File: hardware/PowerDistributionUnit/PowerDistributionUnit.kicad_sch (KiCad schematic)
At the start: 52 parts, among them J1 973582101, J2 973582100, J3 973582101, J4 973582100, Q16 CSD18511Q5A, U1 TPS25983, U2 AD5258

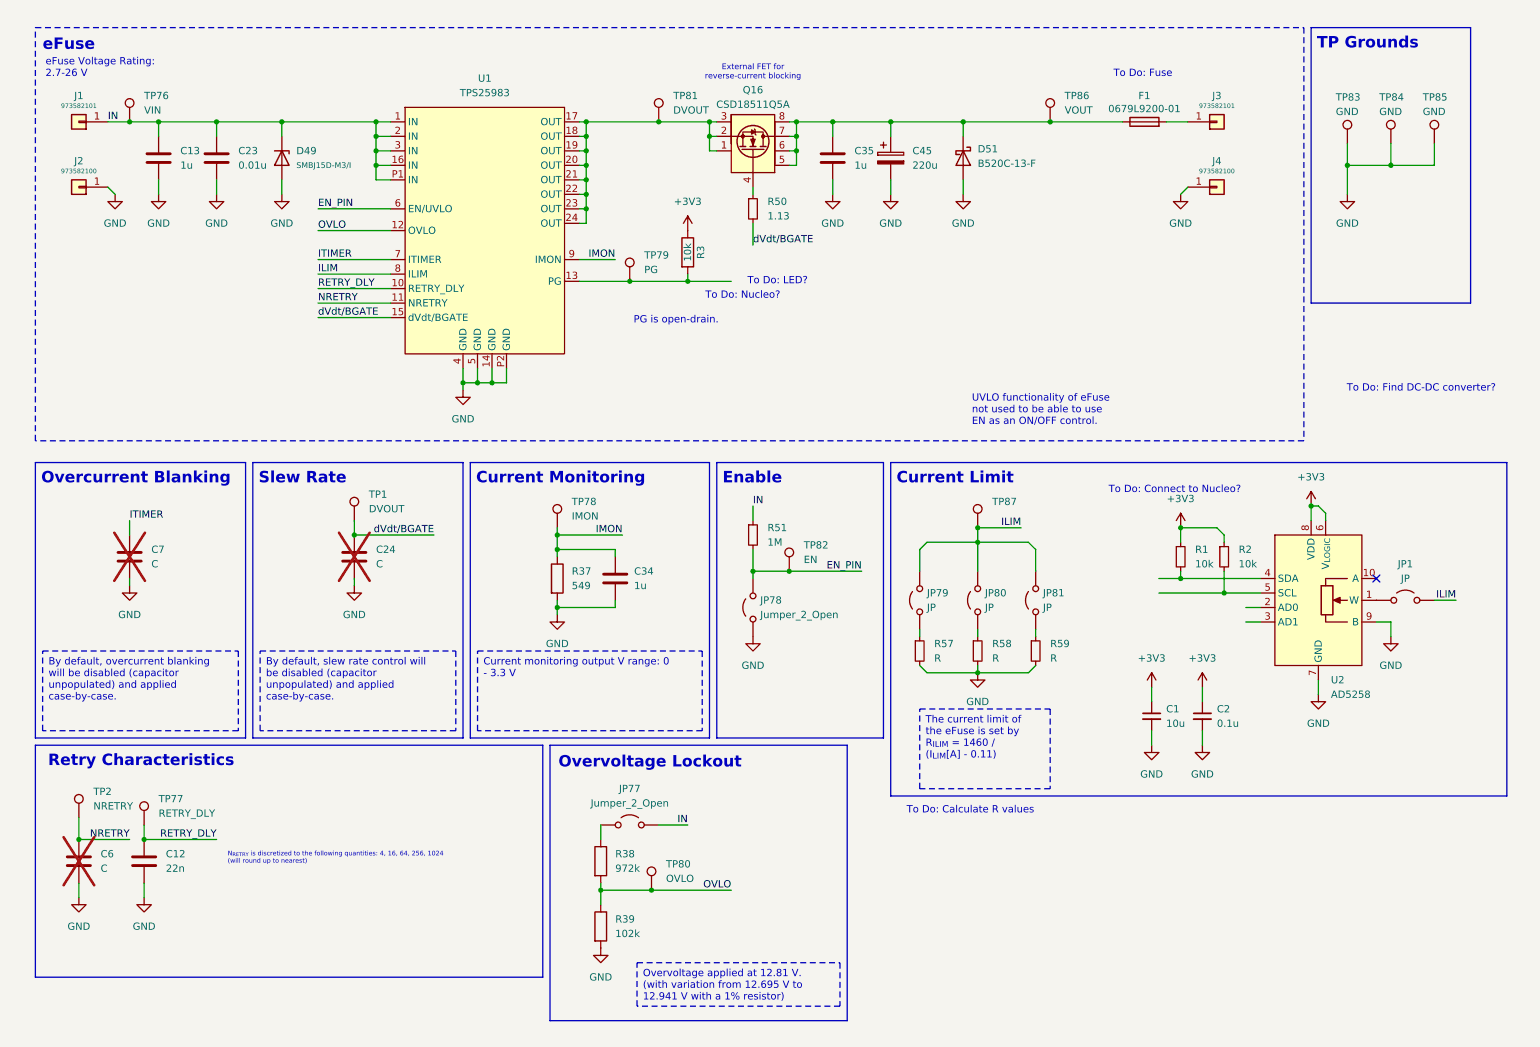
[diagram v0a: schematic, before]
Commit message: schematic work
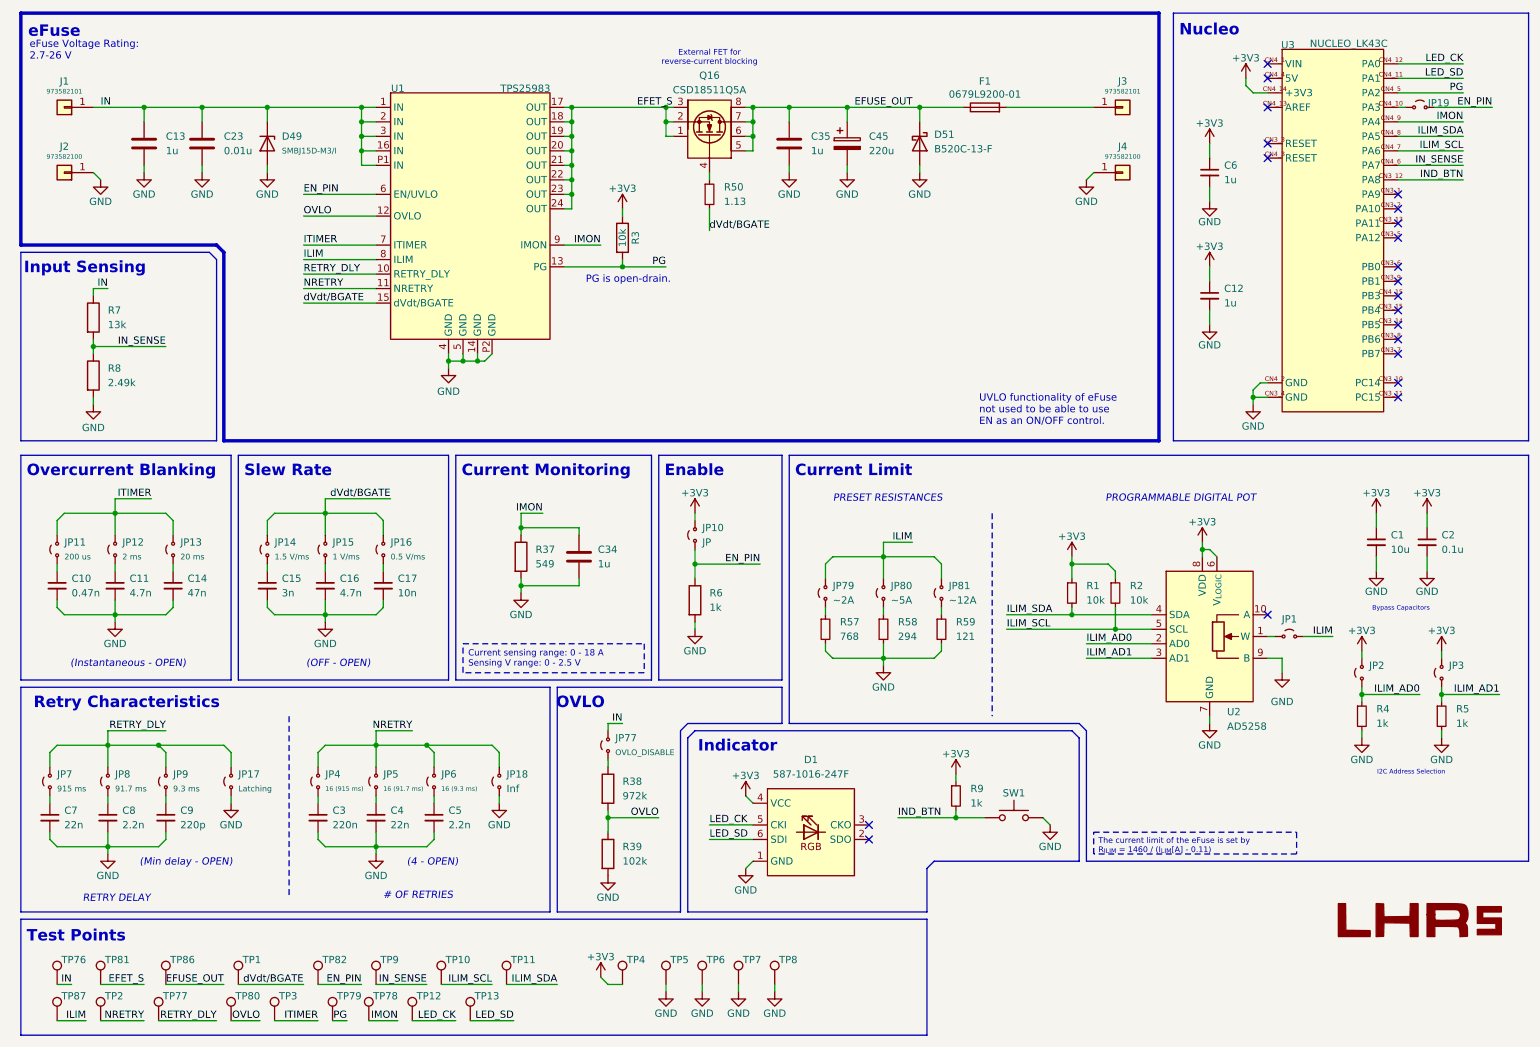
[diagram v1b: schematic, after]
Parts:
- removed C12: 22n, symbol Device:C
- removed C24, C6, C7: C, symbol Device:C
- removed JP78: Jumper_2_Open, symbol Jumper:Jumper_2_Open
- removed R51: 1M, symbol Device:R_Small
- removed TP83, TP84, TP85: GND, symbol Connector:TestPoint
- added C10: 0.47n, symbol Device:C_Small
- added C11, C16: 4.7n, symbol Device:C_Small
- added C12, C6: 1u, symbol Device:C_Small
- added C14: 47n, symbol Device:C_Small
- added C15: 3n, symbol Device:C_Small
- added C17: 10n, symbol Device:C_Small
- added C3: 220n, symbol Device:C_Small
- added C4, C7: 22n, symbol Device:C_Small
- added C5, C8: 2.2n, symbol Device:C_Small
- added C9: 220p, symbol Device:C_Small
- added D1: 587-1016-247F, PowerDistributionUnitLib:587-1016-247F, symbol PowerDistributionUnitLib:587-1016-247F
- added JP10, JP19: JP, symbol Jumper:Jumper_2_Small_Open
- added JP11: 200 us, symbol Jumper:Jumper_2_Small_Open
- added JP12: 2 ms, symbol Jumper:Jumper_2_Small_Open
- added JP13: 20 ms, symbol Jumper:Jumper_2_Small_Open
- added JP14: 1.5 V/ms, symbol Jumper:Jumper_2_Small_Open
- added JP15: 1 V/ms, symbol Jumper:Jumper_2_Small_Open
- added JP16: 0.5 V/ms, symbol Jumper:Jumper_2_Small_Open
- added JP17: Latching, symbol Jumper:Jumper_2_Small_Open
- added JP18: Inf, symbol Jumper:Jumper_2_Small_Open
- added JP2, JP3: Jumper_2_Small_Open, symbol Jumper:Jumper_2_Small_Open
- added JP4: 16 (915 ms), symbol Jumper:Jumper_2_Small_Open
- added JP5: 16 (91.7 ms), symbol Jumper:Jumper_2_Small_Open
- added JP6: 16 (9.3 ms), symbol Jumper:Jumper_2_Small_Open
- added JP7: 915 ms, symbol Jumper:Jumper_2_Small_Open
- added JP8: 91.7 ms, symbol Jumper:Jumper_2_Small_Open
- added JP9: 9.3 ms, symbol Jumper:Jumper_2_Small_Open
- added R4, R5, R9: 1k, symbol Device:R_Small
- added R6: 1k, symbol Device:R
- added R7: 13k, symbol Device:R
- added R8: 2.49k, symbol Device:R
- added SW1: SW_Push, Button_Switch_SMD:SW_SPST_PTS645, symbol Switch:SW_Push
- added TP10, TP11, TP12, TP13, TP9: VIN, symbol Connector:TestPoint
- added TP3: ITIMER, symbol Connector:TestPoint
- added TP4: 3.3V, symbol Connector:TestPoint
- added TP5, TP6, TP7, TP8: GND, symbol Connector:TestPoint
- added U3: NUCLEO_LK43C, symbol PowerDistributionUnitLib:NUCLEO_L43KC
- JP1: symbol Jumper:Jumper_2_Open -> Jumper:Jumper_2_Small_Open
- JP77: value Jumper_2_Open -> OVLO_DISABLE; symbol Jumper:Jumper_2_Open -> Jumper:Jumper_2_Small_Open
- JP79: value JP -> ~2A; symbol Jumper:Jumper_2_Open -> Jumper:Jumper_2_Small_Open
- JP80: value JP -> ~5A; symbol Jumper:Jumper_2_Open -> Jumper:Jumper_2_Small_Open
- JP81: value JP -> ~12A; symbol Jumper:Jumper_2_Open -> Jumper:Jumper_2_Small_Open
- R57: value R -> 768
- R58: value R -> 294
- R59: value R -> 121
- TP81: value DVOUT -> EFET_S
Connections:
- net +3V3: now also C12.1, C6.1, D1.4 (VCC), JP10.2 (B), JP2.2 (B), JP3.2 (B), R9.1, TP4.1, U3.CN4_14 (+3V3)
- net EN_PIN: now also JP10.1 (A), JP19.2 (B), R6.1
- net GND: now also C10.2, C11.2, C12.2, C14.2, C15.2, C16.2, C17.2, C3.2, C4.2, C5.2, C6.2, C7.2, C8.2, C9.2, D1.1 (GND), JP17.1 (A), JP18.1 (A), R4.2, R5.2, R6.2, R8.2, SW1.2, TP5.1, TP6.1, TP7.1, TP8.1, U3.CN3_4 (GND), U3.CN4_2 (GND)
- net IMON: now also U3.CN4_9 (PA4)
- net IN: now also R7.1
- net ITIMER: now also JP11.2 (B), JP12.2 (B), JP13.2 (B), TP3.1
- net NRETRY: now also JP18.2 (B), JP4.2 (B), JP5.2 (B), JP6.2 (B)
- net RETRY_DLY: now also JP17.2 (B), JP7.2 (B), JP8.2 (B), JP9.2 (B)
- net dVdt/BGATE: now also JP14.2 (B), JP15.2 (B), JP16.2 (B)
- net EFUSE_OUT: now reaches C35.1, C45.1, D51.1 (K), F1.1, Q16.5, Q16.6, Q16.7, Q16.8, TP86.1
- net EFET_S: now reaches Q16.1, Q16.2, Q16.3, TP81.1, U1.17 (OUT), U1.18 (OUT), U1.19 (OUT), U1.20 (OUT), U1.21 (OUT), U1.22 (OUT), U1.23 (OUT), U1.24 (OUT)
- net PG: now reaches R3.2, TP79.1, U1.13 (PG)
- net PG: now also U3.CN4_5 (PA2)
- net ILIM_SCL: now reaches R2.2, U2.5 (SCL)
- net ILIM_SCL: now also TP10.1, U3.CN4_7 (PA6)
- net ILIM_AD0: now reaches U2.2 (AD0)
- net ILIM_AD0: now also JP2.1 (A), R4.1
- net ILIM_AD1: now reaches U2.3 (AD1)
- net ILIM_AD1: now also JP3.1 (A), R5.1
- net ILIM_SDA: now reaches R1.2, U2.4 (SDA)
- net ILIM_SDA: now also TP11.1, U3.CN4_8 (PA5)
- new net: C4.1, JP5.1 (A)
- new net: C17.1, JP16.1 (A)
- new net: C15.1, JP14.1 (A)
- new net: C9.1, JP9.1 (A)
- new net: C5.1, JP6.1 (A)
- new net: C3.1, JP4.1 (A)
- new net: C10.1, JP11.1 (A)
- new net: C16.1, JP15.1 (A)
- new net: C11.1, JP12.1 (A)
- new net: C8.1, JP8.1 (A)
- new net: C7.1, JP7.1 (A)
- new net: C14.1, JP13.1 (A)
- new net: JP19.1 (A), U3.CN4_10 (PA3)
- new net IND_BTN: R9.2, SW1.1, U3.CN3_12 (PA8)
- new net IN_SENSE: R7.2, R8.1, TP9.1, U3.CN4_6 (PA7)
- new net LED_CK: D1.5 (CKI), TP12.1, U3.CN4_12 (PA0)
- new net LED_SD: D1.6 (SDI), TP13.1, U3.CN4_11 (PA1)
- no-connect marks 1 -> 21
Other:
- note added: "# OF RETRIES"
- note added: "(4 - OPEN)"
- note added: "(Instantaneous - OPEN)"
- note added: "(Min delay - OPEN)"
- note added: "(OFF - OPEN)"
- note added: "Bypass Capacitors"
- note added: "I2C Address Selection"
- note added: "Indicator"
- note added: "Input Sensing"
- note added: "Nucleo"
- note added: "OVLO"
- note added: "PRESET RESISTANCES"
- note added: "PROGRAMMABLE DIGITAL POT"
- note added: "RETRY DELAY"
- note added: "Test Points"
- note removed: "Overvoltage Lockout"
- note removed: "TP Grounds"
- note removed: "To Do: Calculate R values"
- note removed: "To Do: Connect to Nucleo?"
- note removed: "To Do: Find DC-DC converter?"
- note removed: "To Do: Fuse"
- note removed: "To Do: LED?"
- note removed: "To Do: Nucleo?"
- company: (none) -> Longhorn Racing: Solar
- title: (none) -> eFuse Test Board
- moved on the sheet: C1, C13, C2, C23, C34, C35, C45, D49, D51, F1, J1, J2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
